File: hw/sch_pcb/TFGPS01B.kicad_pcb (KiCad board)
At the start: 4 copper layers, 51 x 51 mm, 72 parts, among them J1 SM10B-GHS-TB, J2 USBC_USB4105-GF-A, J3 SM06B-GHS-TB, J4 SM04B-GHS-TB, J5 SM08B-GHS-TB, M1 HOLE, M2 HOLE, M3 HOLE, M4 HOLE, Q1 BC817-25, Q2 BC817-25, Q3 BC817-25, U1 MIC5504-3.3YM5, U2 USBLC6-2SC6, U3 NEO-M8P, U4 MAX2655

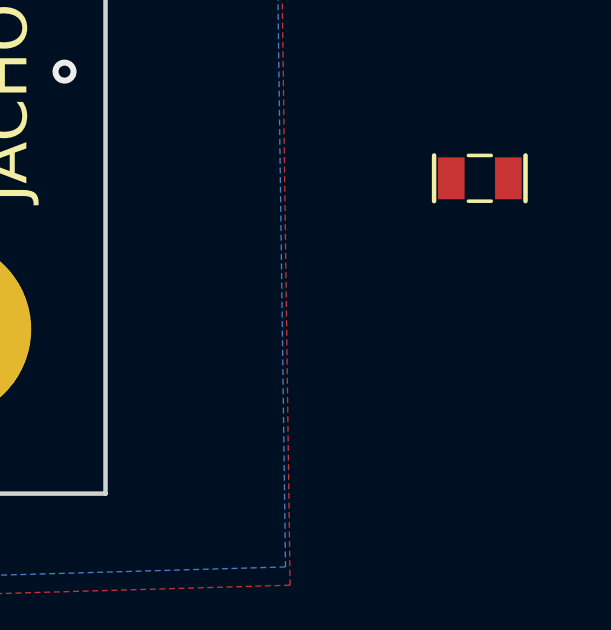
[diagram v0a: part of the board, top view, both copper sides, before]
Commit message: Edit schema
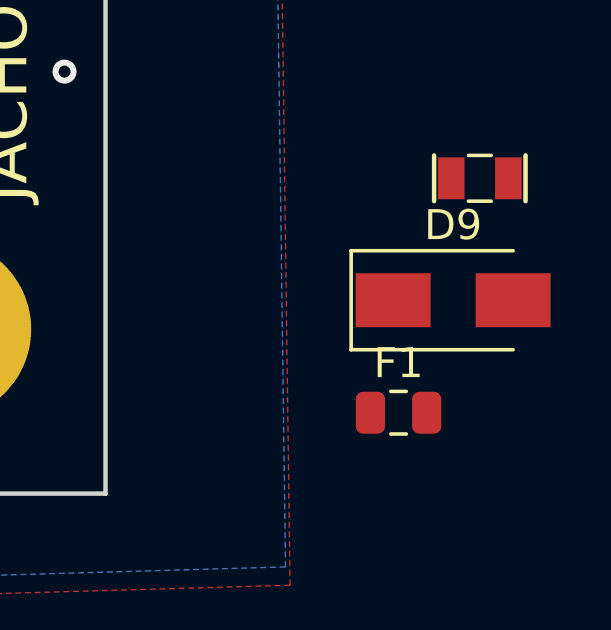
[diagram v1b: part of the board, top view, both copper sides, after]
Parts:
- added D9: 15MQ040N, Diode_SMD:D_SMA, F.Cu at (62.5, -6.35)
- added F1: 750mA, Fuse:Fuse_0805_2012Metric, F.Cu at (60.7, -2.60)
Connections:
- J2 pad A4/B9: +5V -> /VBUS
- J2 pad B4/A9: +5V -> /VBUS
- U2 pad 5: +5V -> /VBUS
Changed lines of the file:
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@@
   (net 64 "unconnected-(U3-Pad14)")
   (net 65 "unconnected-(U3-Pad17)")
+  (net 66 "Net-(D9-Pad2)")
+  (net 67 "/VBUS")
   (footprint "Mlab_Mechanical:MountingHole_3mm" placed (layer "F.Cu")
     (at 45.42 -5.38)
@@
       (net 1 "GND") (pintype "input") (clearance 1) (zone_connect 2))
     (model "${MLAB}/src/3d/mechanical/m3_komplet.step"
+      (offset (xyz 0 0 0))
+      (scale (xyz 1 1 1))
+      (rotate (xyz 0 0 0))
+    )
+  )
+  (footprint "Fuse:Fuse_0805_2012Metric" (layer "F.Cu")
+    (at 60.664 -2.6)
+    (descr "Fuse SMD 0805 (2012 Metric), square (rectangular) end terminal, IPC_7351 nominal, (Body size source: https://docs.google.com/spreadsheets/d/1BsfQQcO9C6DZCsRaXUlFlo91Tg2WpOkGARC1WS5S8t0/edit?usp=sharing), generated with kicad-footprint-generator")
+    (tags "fuse")
+    (property "Sheetfile" "TFGPS01B.kicad_sch")
+    (property "Sheetname" "")
+    (attr smd)
+    (fp_text reference "F1" (at 0 -1.65) (layer "F.SilkS")
+      (effects (font (size 1 1) (thickness 0.15)))
+    )
+    (fp_text value "750mA" (at 0 1.65) (layer "F.Fab")
+      (effects (font (size 1 1) (thickness 0.15)))
+    )
+    (fp_text user "${REFERENCE}" (at 0 0) (layer "F.Fab")
+      (effects (font (size 0.5 0.5) (thickness 0.08)))
+    )
+    (fp_line (start -0.258578 0.71) (end 0.258578 0.71) (layer "F.SilkS") (width 0.12))
+    (fp_line (start -0.258578 -0.71) (end 0.258578 -0.71) (layer "F.SilkS") (width 0.12))
+    (fp_line (start 1.68 -0.95) (end 1.68 0.95) (layer "F.CrtYd") (width 0.05))
+    (fp_line (start 1.68 0.95) (end -1.68 0.95) (layer "F.CrtYd") (width 0.05))
+    (fp_line (start -1.68 0.95) (end -1.68 -0.95) (layer "F.CrtYd") (width 0.05))
+    (fp_line (start -1.68 -0.95) (end 1.68 -0.95) (layer "F.CrtYd") (width 0.05))
+    (fp_line (start 1 -0.6) (end 1 0.6) (layer "F.Fab") (width 0.1))
+    (fp_line (start 1 0.6) (end -1 0.6) (layer "F.Fab") (width 0.1))
+    (fp_line (start -1 -0.6) (end 1 -0.6) (layer "F.Fab") (width 0.1))
+    (fp_line (start -1 0.6) (end -1 -0.6) (layer "F.Fab") (width 0.1))
+    (pad "1" smd roundrect locked (at -0.9375 0) (size 0.975 1.4) (layers "F.Cu" "F.Paste" "F.Mask") (roundrect_rratio 0.25)
+      (net 67 "/VBUS") (pintype "passive"))
+    (pad "2" smd roundrect locked (at 0.9375 0) (size 0.975 1.4) (layers "F.Cu" "F.Paste" "F.Mask") (roundrect_rratio 0.25)
+      (net 66 "Net-(D9-Pad2)") (pintype "passive"))
+    (model "${KISYS3DMOD}/Fuse.3dshapes/Fuse_0805_2012Metric.wrl"
       (offset (xyz 0 0 0))
       (scale (xyz 1 1 1))
@@
       (net 57 "/SAFE_VCC") (pintype "passive"))
     (model "${KISYS3DMOD}/Resistor_SMD.3dshapes/R_0805_2012Metric.wrl"
+      (offset (xyz 0 0 0))
+      (scale (xyz 1 1 1))
+      (rotate (xyz 0 0 0))
+    )
+  )
+  (footprint "Diode_SMD:D_SMA" (layer "F.Cu")
+    (at 62.484 -6.35)
+    (descr "Diode SMA (DO-214AC)")
+    (tags "Diode SMA (DO-214AC)")
+    (property "Sheetfile" "TFGPS01B.kicad_sch")
+    (property "Sheetname" "")
+    (property "UST_ID" "5c70984512875079b91f88b0")
+    (attr smd)
+    (fp_text reference "D9" (at 0 -2.5) (layer "F.SilkS")
+      (effects (font (size 1 1) (thickness 0.15)))
+    )
+    (fp_text value "15MQ040N" (at 0 2.6) (layer "F.Fab")
+      (effects (font (size 1 1) (thickness 0.15)))
+    )
+    (fp_text user "${REFERENCE}" (at 0 -2.5) (layer "F.Fab")
+      (effects (font (size 1 1) (thickness 0.15)))
+    )
+    (fp_line (start -3.4 1.65) (end 2 1.65) (layer "F.SilkS") (width 0.12))
+    (fp_line (start -3.4 -1.65) (end -3.4 1.65) (layer "F.SilkS") (width 0.12))
+    (fp_line (start -3.4 -1.65) (end 2 -1.65) (layer "F.SilkS") (width 0.12))
+    (fp_line (start -3.5 -1.75) (end 3.5 -1.75) (layer "F.CrtYd") (width 0.05))
+    (fp_line (start -3.5 1.75) (end -3.5 -1.75) (layer "F.CrtYd") (width 0.05))
+    (fp_line (start 3.5 1.75) (end -3.5 1.75) (layer "F.CrtYd") (width 0.05))
+    (fp_line (start 3.5 -1.75) (end 3.5 1.75) (layer "F.CrtYd") (width 0.05))
+    (fp_line (start 2.3 1.5) (end -2.3 1.5) (layer "F.Fab") (width 0.1))
+    (fp_line (start 0.50118 0.00102) (end 1.4994 0.00102) (layer "F.Fab") (width 0.1))
+    (fp_line (start 2.3 -1.5) (end -2.3 -1.5) (layer "F.Fab") (width 0.1))
+    (fp_line (start -2.3 1.5) (end -2.3 -1.5) (layer "F.Fab") (width 0.1))
+    (fp_line (start -0.64944 0.00102) (end 0.50118 0.75032) (layer "F.Fab") (width 0.1))
+    (fp_line (start -0.64944 0.00102) (end 0.50118 -0.79908) (layer "F.Fab") (width 0.1))
+    (fp_line (start -0.64944 0.00102) (end -1.55114 0.00102) (layer "F.Fab") (width 0.1))
+    (fp_line (start 2.3 -1.5) (end 2.3 1.5) (layer "F.Fab") (width 0.1))
+    (fp_line (start 0.50118 0.75032) (end 0.50118 -0.79908) (layer "F.Fab") (width 0.1))
+    (fp_line (start -0.64944 -0.79908) (end -0.64944 0.80112) (layer "F.Fab") (width 0.1))
+    (pad "1" smd rect locked (at -2 0) (size 2.5 1.8) (layers "F.Cu" "F.Paste" "F.Mask")
+      (net 7 "+5V") (pinfunction "K") (pintype "passive"))
+    (pad "2" smd rect locked (at 2 0) (size 2.5 1.8) (layers "F.Cu" "F.Paste" "F.Mask")
+      (net 66 "Net-(D9-Pad2)") (pinfunction "A") (pintype "passive"))
+    (model "${KISYS3DMOD}/Diode_SMD.3dshapes/D_SMA.wrl"
       (offset (xyz 0 0 0))
       (scale (xyz 1 1 1))
@@
       (net 12 "/D-") (pinfunction "IO2") (pintype "passive"))
     (pad "5" smd rect locked (at 1.1 0 180) (size 1.06 0.65) (layers "B.Cu" "B.Paste" "B.Mask")
-      (net 7 "+5V") (pinfunction "VBUS") (pintype "passive"))
+      (net 67 "/VBUS") (pinfunction "VBUS") (pintype "passive"))
     (pad "6" smd rect locked (at 1.1 0.95 180) (size 1.06 0.65) (layers "B.Cu" "B.Paste" "B.Mask")
       (net 11 "/D+") (pinfunction "IO1") (pintype "passive"))
@@
       (net 1 "GND") (pinfunction "GND") (pintype "passive"))
     (pad "A4/B9" smd rect locked (at -2.4 4.755 90) (size 0.6 1.15) (layers "B.Cu" "B.Paste" "B.Mask")
-      (net 7 "+5V") (pinfunction "VBUS") (pintype "passive"))
+      (net 67 "/VBUS") (pinfunction "VBUS") (pintype "passive"))
     (pad "A5" smd rect locked (at -1.25 4.755 90) (size 0.3 1.15) (layers "B.Cu" "B.Paste" "B.Mask")
       (net 40 "Net-(J2-PadA5)") (pinfunction "CC1") (pintype "bidirectional"))
@@
       (net 1 "GND") (pinfunction "GND") (pintype "passive"))
     (pad "B4/A9" smd rect locked (at 2.4 4.755 90) (size 0.6 1.15) (layers "B.Cu" "B.Paste" "B.Mask")
-      (net 7 "+5V") (pinfunction "VBUS") (pintype "passive"))
+      (net 67 "/VBUS") (pinfunction "VBUS") (pintype "passive"))
     (pad "B5" smd rect locked (at 1.75 4.755 90) (size 0.3 1.15) (layers "B.Cu" "B.Paste" "B.Mask")
       (net 41 "Net-(J2-PadB5)") (pinfunction "CC2") (pintype "bidirectional"))
